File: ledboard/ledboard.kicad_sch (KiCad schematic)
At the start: 45 parts, among them J1 Jack-DC, U1 TPS54332DDA, U2 TPS7A5301BRPSR, U3 TPS2121

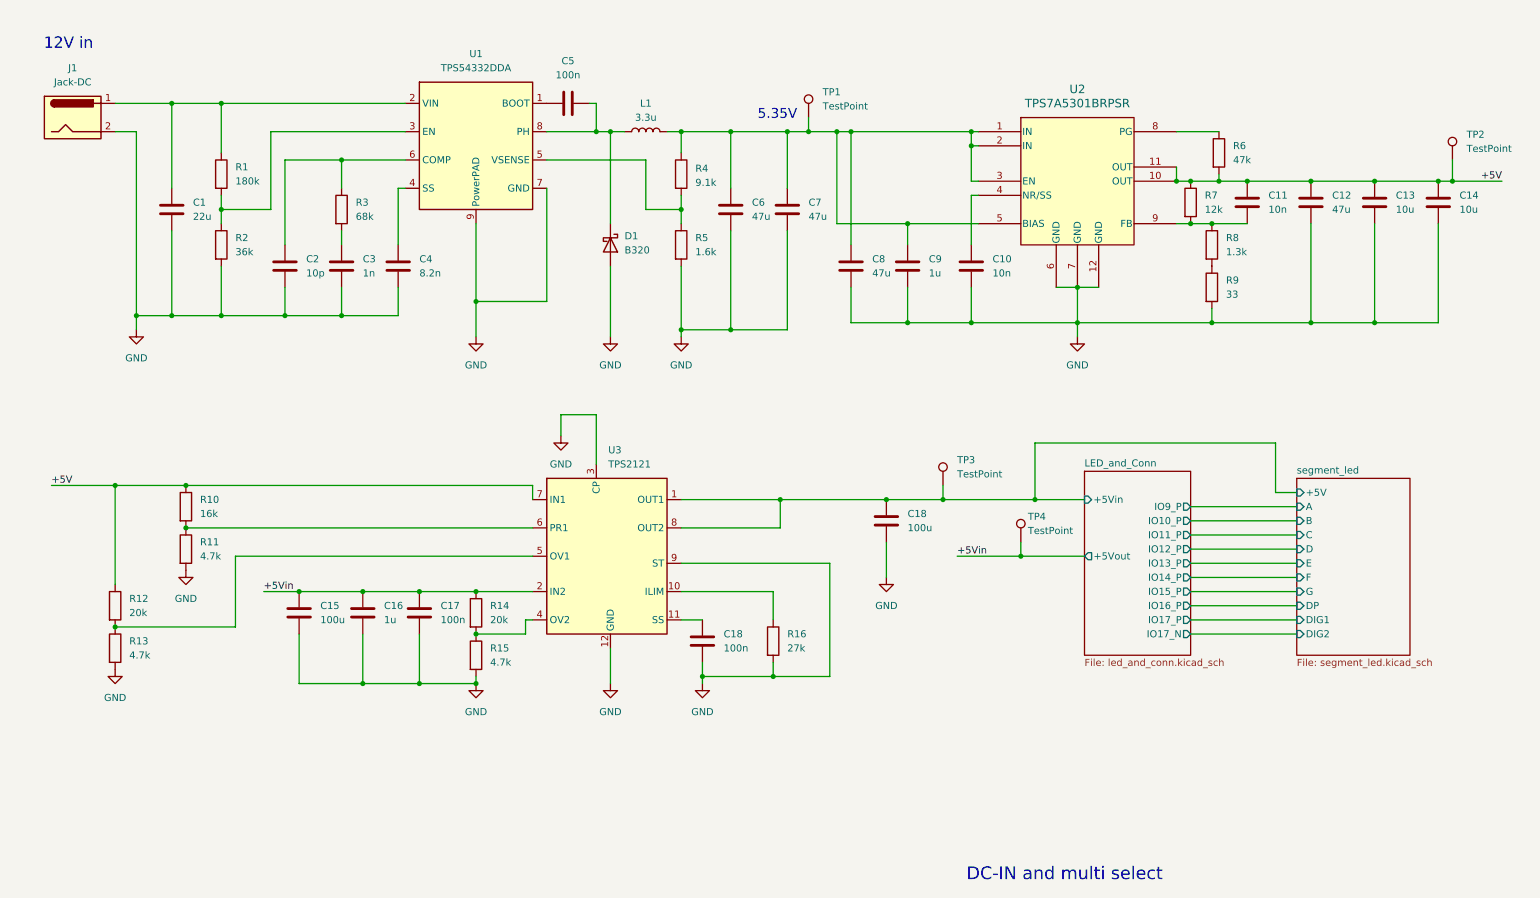
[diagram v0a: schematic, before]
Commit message: 部品が決まったので,コミットします.
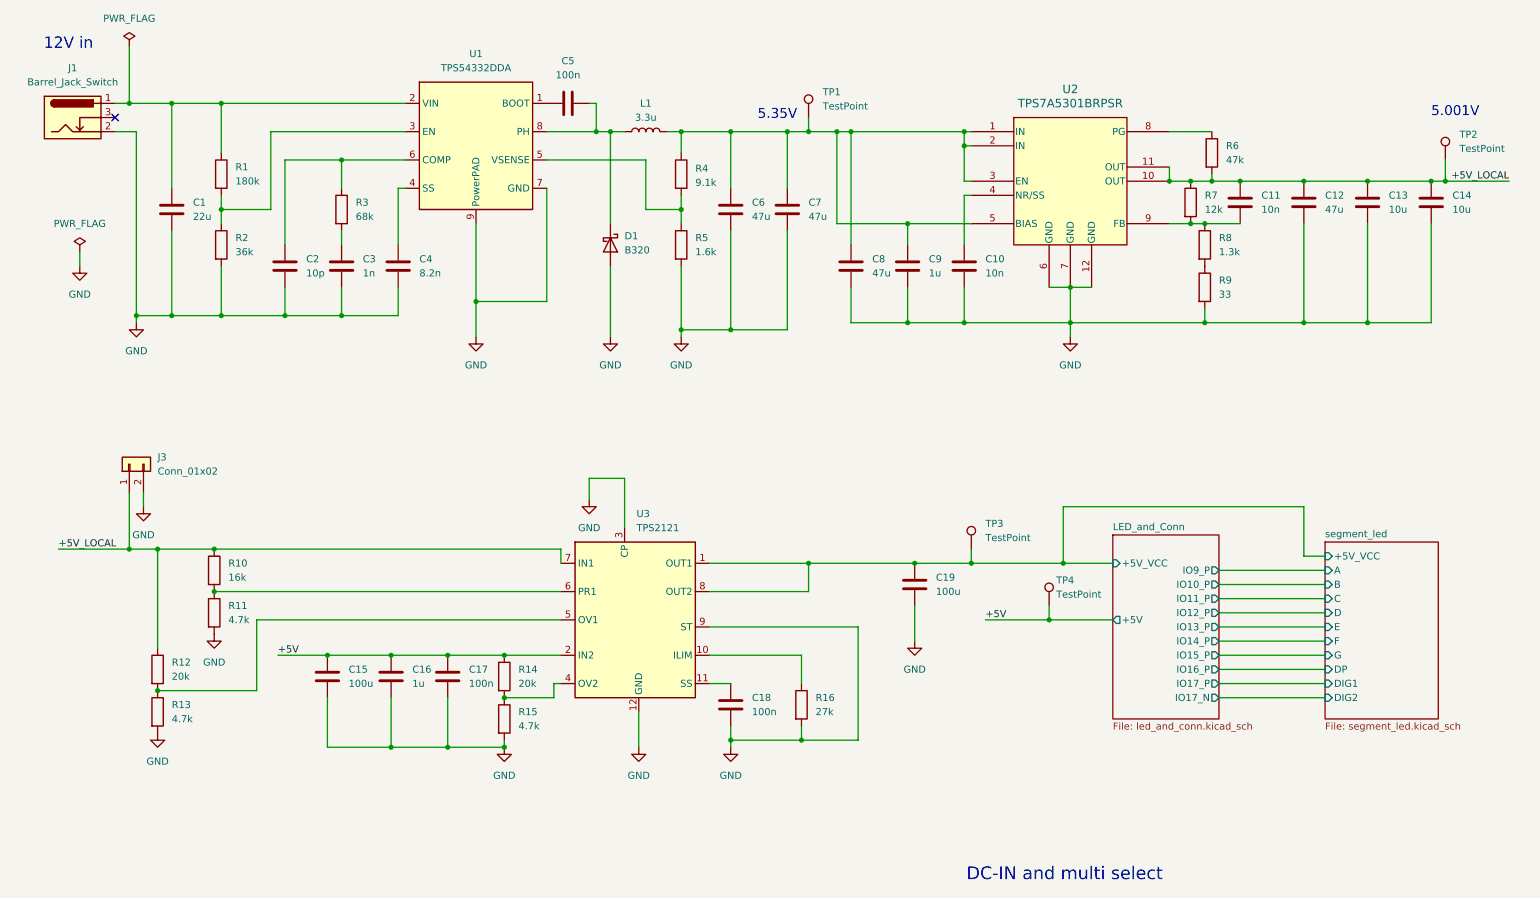
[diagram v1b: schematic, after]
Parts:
- removed J1: Jack-DC, symbol Connector:Jack-DC
- added J1: Barrel_Jack_Switch, MyLib:MPD_EJ503A, symbol Connector:Barrel_Jack_Switch
- added J3: Conn_01x02, Connector_PinHeader_2.54mm:PinHeader_1x02_P2.54mm_Vertical, symbol Connector_Generic:Conn_01x02
- C10: footprint Capacitor_SMD:C_1206_3216Metric -> Capacitor_SMD:C_01005_0402Metric; MPN GRM31CR61C476ME44 -> GRM022R61C103ME01
- C11: footprint (none) -> Capacitor_SMD:C_01005_0402Metric; MPN (none) -> GRM022R61C103ME01; Manufacturer (none) -> Murata
- C12: footprint (none) -> Capacitor_SMD:C_1206_3216Metric; MPN (none) -> GRM31CR61C476ME44; Manufacturer (none) -> Murata
- C13, C14: footprint (none) -> Capacitor_SMD:C_0603_1608Metric; MPN (none) -> GRM188R61C106MA73; Manufacturer (none) -> Murata
- C15: footprint (none) -> Capacitor_SMD:C_1210_3225Metric; MPN (none) -> GRM32ER61A107ME20; Manufacturer (none) -> Murata
- C16: footprint (none) -> Capacitor_SMD:C_0402_1005Metric; MPN (none) -> GRM155C71A105KE11; Manufacturer (none) -> Murata
- C17, C18: footprint (none) -> Capacitor_SMD:C_0201_0603Metric; MPN (none) -> GRM033C81A104ME14; Manufacturer (none) -> Murata
- C19: renamed from C18; footprint (none) -> Capacitor_SMD:C_1210_3225Metric; MPN (none) -> GRM32ER61A107ME20; Manufacturer (none) -> Murata
- C2: MPN GRM1555C2A100JA01 -> GRM0222C1C100JA03
- C3: footprint (none) -> Capacitor_SMD:C_0201_0603Metric; MPN (none) -> GRM033R71C102KA01; Manufacturer (none) -> Murata
- C4: footprint (none) -> Capacitor_SMD:C_0201_0603Metric; MPN (none) -> GRM033B11A822JA01; Manufacturer (none) -> Murata
- C5: footprint (none) -> Capacitor_SMD:C_0201_0603Metric; MPN (none) -> GRM033C81E104ME14; Manufacturer (none) -> Murata
- C9: footprint Capacitor_SMD:C_1206_3216Metric -> Capacitor_SMD:C_0402_1005Metric; MPN GRM31CR61C476ME44 -> GRM155B31C105KA12
- L1: footprint (none) -> MyLib:SPM7054VC-3R3M-D
- R1: MPN (none) -> RC0603FR-07180KL; Manufacturer (none) -> YAGEO
- R10: footprint (none) -> Resistor_SMD:R_0603_1608Metric; MPN (none) -> RC0603FR-0716KL; Manufacturer (none) -> YAGEO
- R11, R13, R15: footprint (none) -> Resistor_SMD:R_0603_1608Metric; MPN (none) -> RC0603FR-074K7L; Manufacturer (none) -> YAGEO
- R12, R14: footprint (none) -> Resistor_SMD:R_0603_1608Metric; MPN (none) -> RC0603FR-0720KL; Manufacturer (none) -> YAGEO
- R16: footprint (none) -> Resistor_SMD:R_0603_1608Metric; MPN (none) -> RC0603FR-0727KL; Manufacturer (none) -> YAGEO
- R2: MPN (none) -> RC0603FR-0736KL; Manufacturer (none) -> YAGEO
- R3: footprint (none) -> Resistor_SMD:R_0603_1608Metric; MPN (none) -> RC0603FR-0768KL; Manufacturer (none) -> YAGEO
- R4: footprint (none) -> Resistor_SMD:R_0603_1608Metric; MPN (none) -> RC0603FR-0769K1L; Manufacturer (none) -> YAGEO
- R5: footprint (none) -> Resistor_SMD:R_0603_1608Metric; MPN (none) -> RC0603FR-071K6L; Manufacturer (none) -> YAGEO
- R6: footprint (none) -> Resistor_SMD:R_0603_1608Metric; MPN (none) -> RC0603FR-0747KL; Manufacturer (none) -> YAGEO
- R7: footprint (none) -> Resistor_SMD:R_0603_1608Metric; MPN (none) -> RC0603FR-0712KL; Manufacturer (none) -> YAGEO
- R8: footprint (none) -> Resistor_SMD:R_0603_1608Metric; MPN (none) -> RC0603FR-071K3L; Manufacturer (none) -> YAGEO
- R9: footprint (none) -> Resistor_SMD:R_0603_1608Metric; MPN (none) -> RC0603FR-0733RL; Manufacturer (none) -> YAGEO
- TP1, TP2, TP3, TP4: footprint (none) -> TestPoint:TestPoint_Keystone_5000-5004_Miniature; MPN (none) -> 5002; Manufacturer (none) -> keystone
- U2: MPN (none) -> TPS7A5301BRPSR; Manufacturer (none) -> TI
- U3: MPN TPS2121 -> TPS2121RUXR
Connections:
- net +5Vin is gone; now on net +5V: C15.1, C16.1, C17.1, R14.1, TP4.1, U3.2 (IN2)
- net +5V: no longer C11.1, C12.1, C13.1, C14.1, R10.1, R12.1, R6.2, R7.1, TP2.1, U2.10 (OUT), U2.11 (OUT), U3.7 (IN1)
- net GND: now also J1.2, J3.2 (Pin_2)
- net at C1.1, R1.1, U1.2 (VIN): now also J1.1
- net LED_and_Conn/+5Vin renamed LED_and_Conn/+5V_VCC
- new net +5V_LOCAL: C11.1, C12.1, C13.1, C14.1, J3.1 (Pin_1), R10.1, R12.1, R6.2, R7.1, TP2.1, U2.10 (OUT), U2.11 (OUT), U3.7 (IN1)
- no-connect marks 0 -> 1
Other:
- sheet LED_and_Conn ports: added +5V, +5V_VCC; removed +5Vin, +5Vout
- sheet segment_led ports: added +5V_VCC; removed +5V
- note added: "5.001V"
- moved on the sheet: C10, C11, C12, C13, C14, C15, C16, C17, C18, C19, R10, R11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

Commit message: ERC解消まで.
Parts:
- U3: MPN TPS2121RUXR -> TPS2121
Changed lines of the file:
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@@
 			)
 		)
-		(property "Datasheet" "https://pim.murata.com/asset/pim4/ceramicCapacitorSMD/GRM022R61E103ME01-01A-JP_PDF_CERAMICCAPACITORSMD?lastModifiedDatetime=20250813135319"
+		(property "Datasheet" "~"
 			(at 233.68 52.07 0)
 			(effects
@@
 			)
 		)
-		(property "Datasheet" "https://www.memoryprotectiondevices.com/datasheets/EJ503A/EJ503A-datasheet.pdf"
+		(property "Datasheet" "~"
 			(at 25.4 37.846 0)
 			(effects
@@
 			)
 		)
-		(property "Datasheet" "https://yageogroup.com/content/datasheet/asset/file/PYU-RC_GROUP_51_ROHS_L"
+		(property "Datasheet" "~"
 			(at 39.37 143.51 0)
 			(effects
@@
 			)
 		)
-		(property "Datasheet" "https://pim.murata.com/asset/pim4/ceramicCapacitorSMD/GRM033B11A222JA01-01A-JP_PDF_CERAMICCAPACITORSMD?lastModifiedDatetime=20250813141149"
+		(property "Datasheet" "~"
 			(at 82.55 63.5 0)
 			(effects
@@
 			)
 		)
-		(property "Datasheet" "https://pim.murata.com/asset/pim4/ceramicCapacitorSMD/GRM155B31C105KA12-01A-JP_PDF_CERAMICCAPACITORSMD?lastModifiedDatetime=20250813144309"
+		(property "Datasheet" "~"
 			(at 173.99 63.5 0)
 			(effects
@@
 			)
 		)
-		(property "Datasheet" "https://pim.murata.com/asset/pim4/ceramicCapacitorSMD/GRM033R71C102KA01-01A-JP_PDF_CERAMICCAPACITORSMD?lastModifiedDatetime=20250813141657"
+		(property "Datasheet" "~"
 			(at 72.39 63.5 0)
 			(effects
@@
 			)
 		)
-		(property "Datasheet" "https://www.keyelco.com/userAssets/file/K75p62.pdf"
+		(property "Datasheet" "~"
 			(at 275.59 44.45 0)
 			(effects
@@
 			)
 		)
-		(property "Datasheet" "https://pim.murata.com/asset/pim4/ceramicCapacitorSMD/GRM033C81A104ME14-01A-JP_PDF_CERAMICCAPACITORSMD?lastModifiedDatetime=20250813141354"
+		(property "Datasheet" "~"
 			(at 142.24 142.24 0)
 			(effects
@@
 			)
 		)
-		(property "Datasheet" "https://yageogroup.com/content/datasheet/asset/file/PYU-RC_GROUP_51_ROHS_L"
+		(property "Datasheet" "~"
 			(at 228.6 43.18 0)
 			(effects
@@
 			)
 		)
-		(property "Datasheet" "https://pim.murata.com/asset/pim4/ceramicCapacitorSMD/GRM32ER61A107ME20-01A-JP_PDF_CERAMICCAPACITORSMD?lastModifiedDatetime=20250813153035"
+		(property "Datasheet" "~"
 			(at 69.85 137.16 0)
 			(effects
@@
 			)
 		)
-		(property "Datasheet" "https://pim.murata.com/asset/pim4/ceramicCapacitorSMD/GRM188R61C106MA73-01A-JP_PDF_CERAMICCAPACITORSMD?lastModifiedDatetime=20250813150719"
+		(property "Datasheet" "~"
 			(at 256.54 52.07 0)
 			(effects
@@
 			)
 		)
-		(property "Datasheet" "https://pim.murata.com/asset/pim4/ceramicCapacitorSMD/GRM022R61E103ME01-01A-JP_PDF_CERAMICCAPACITORSMD?lastModifiedDatetime=20250813135319"
+		(property "Datasheet" "~"
 			(at 184.15 63.5 0)
 			(effects
@@
 			)
 		)
-		(property "Datasheet" "https://www.keyelco.com/userAssets/file/K75p62.pdf"
+		(property "Datasheet" "~"
 			(at 204.47 124.46 0)
 			(effects
@@
 			)
 		)
-		(property "Datasheet" "https://pim.murata.com/asset/pim4/ceramicCapacitorSMD/GRM31CC71E226ME15-01A-JP_PDF_CERAMICCAPACITORSMD?lastModifiedDatetime=20250813152619"
+		(property "Datasheet" "~"
 			(at 41.91 53.34 0)
 			(effects
@@
 			)
 		)
-		(property "Datasheet" "https://yageogroup.com/content/datasheet/asset/file/PYU-RC_GROUP_51_ROHS_L"
+		(property "Datasheet" "~"
 			(at 39.37 135.89 0)
 			(effects
@@
 			)
 		)
-		(property "Datasheet" "https://yageogroup.com/content/datasheet/asset/file/PYU-RC_GROUP_51_ROHS_L"
+		(property "Datasheet" "~"
 			(at 227.33 59.69 0)
 			(effects
@@
 			)
 		)
-		(property "Datasheet" "https://www.keyelco.com/userAssets/file/K75p62.pdf"
+		(property "Datasheet" "~"
 			(at 190.5 114.3 0)
 			(effects
@@
 			)
 		)
-		(property "Datasheet" "https://pim.murata.com/asset/pim4/ceramicCapacitorSMD/GRM188R61C106MA73-01A-JP_PDF_CERAMICCAPACITORSMD?lastModifiedDatetime=20250813150719"
+		(property "Datasheet" "~"
 			(at 267.97 52.07 0)
 			(effects
@@
 			)
 		)
-		(property "Datasheet" "https://pim.murata.com/asset/pim4/ceramicCapacitorSMD/GRM32ER61A107ME20-01A-JP_PDF_CERAMICCAPACITORSMD?lastModifiedDatetime=20250813153035"
+		(property "Datasheet" "~"
 			(at 175.26 120.65 0)
 			(effects
@@
 			)
 		)
-		(property "Datasheet" "https://pim.murata.com/asset/pim4/ceramicCapacitorSMD/GRM31CR61C476ME44-01A-JP_PDF_CERAMICCAPACITORSMD?lastModifiedDatetime=20250813152638"
+		(property "Datasheet" "~"
 			(at 142.24 53.34 0)
 			(effects
@@
 			)
 		)
-		(property "Datasheet" "https://pim.murata.com/asset/pim4/ceramicCapacitorSMD/GRM31CR61C476ME44-01A-JP_PDF_CERAMICCAPACITORSMD?lastModifiedDatetime=20250813152638"
+		(property "Datasheet" "~"
 			(at 152.4 53.34 0)
 			(effects
@@
 			)
 		)
-		(property "Datasheet" "https://pim.murata.com/asset/pim4/ceramicCapacitorSMD/GRM31CR61C476ME44-01A-JP_PDF_CERAMICCAPACITORSMD?lastModifiedDatetime=20250813152638"
+		(property "Datasheet" "~"
 			(at 245.11 52.07 0)
 			(effects
@@
 			)
 		)
-		(property "Datasheet" "https://www.keyelco.com/userAssets/file/K75p62.pdf"
+		(property "Datasheet" "~"
 			(at 161.29 36.83 0)
 			(effects
@@
 			)
 		)
-		(property "Datasheet" "https://yageogroup.com/content/datasheet/asset/file/PYU-RC_GROUP_51_ROHS_L"
+		(property "Datasheet" "~"
 			(at 50.8 59.69 0)
 			(effects
@@
 			)
 		)
-		(property "Datasheet" "https://www.ti.com/jp/lit/ds/symlink/tps54332.pdf?ts=1774599358950&ref_url=https%253A%252F%252Fwww.ti.com%252Fproduct%252Fja-jp%252FTPS54332%253Futm_source%253Dgoogle%2526utm_medium%253Dcpc%2526utm_campaign%253Dapp-null-null-gpn_jp-cpc-pf-google-jp_jp_cons%2526utm_content%253DTPS54332%2526ds_k%253DTPS54332%2526DCM%253Dyes%2526gclsrc%253Daw.ds%2526gad_source%253D1%2526gad_campaignid%253D20279248515%2526gclid%253DCj0KCQjw1ZjOBhCmARIsADDuFTBmD5gUQSDSVcVDqtlcqWftM3LiZUXBOSejrsmSzrKRocTvUMsoHYIaAuFjEALw_wcB"
+		(property "Datasheet" "https://www.ti.com/product/ja-jp/TPS54332#cad-cae-symbols"
 			(at 96.52 41.91 0)
 			(effects
@@
 			)
 		)
-		(property "Description" ""
+		(property "Description" "DC-DC Converter"
 			(at 96.52 41.91 0)
 			(effects
@@
 			)
 		)
-		(property "Datasheet" "https://pim.murata.com/asset/pim4/ceramicCapacitorSMD/GRM155C71A105KE11-01A-JP_PDF_CERAMICCAPACITORSMD?lastModifiedDatetime=20260115145428"
+		(property "Datasheet" "~"
 			(at 81.28 137.16 0)
 			(effects
@@
 			)
 		)
-		(property "Datasheet" "https://yageogroup.com/content/datasheet/asset/file/PYU-RC_GROUP_51_ROHS_L"
+		(property "Datasheet" "~"
 			(at 154.94 142.24 0)
 			(effects
@@
 			)
 		)
-		(property "Datasheet" "https://pim.murata.com/asset/pim4/ceramicCapacitorSMD/GRM033C81A104ME14-01A-JP_PDF_CERAMICCAPACITORSMD?lastModifiedDatetime=20250813141354"
+		(property "Datasheet" "~"
 			(at 91.44 137.16 0)
 			(effects
@@
 			)
 		)
-		(property "Datasheet" "https://pim.murata.com/asset/pim4/ceramicCapacitorSMD/GRM033C81E104ME14-01A-JP_PDF_CERAMICCAPACITORSMD?lastModifiedDatetime=20250813141359"
+		(property "Datasheet" "~"
 			(at 113.03 34.29 0)
 			(effects
@@
 			)
 		)
-		(property "Datasheet" "https://yageogroup.com/content/datasheet/asset/file/PYU-RC_GROUP_51_ROHS_L"
+		(property "Datasheet" "~"
 			(at 101.6 137.16 0)
 			(effects
@@
 			)
 		)
-		(property "Datasheet" "https://yageogroup.com/content/datasheet/asset/file/PYU-RC_GROUP_51_ROHS_L"
+		(property "Datasheet" "~"
 			(at 50.8 46.99 0)
 			(effects
@@
 			)
 		)
-		(property "Datasheet" "https://yageogroup.com/content/datasheet/asset/file/PYU-RC_GROUP_51_ROHS_L"
+		(property "Datasheet" "~"
 			(at 227.33 67.31 0)
 			(effects
@@
 			)
 		)
-		(property "Datasheet" "https://yageogroup.com/content/datasheet/asset/file/PYU-RC_GROUP_51_ROHS_L"
+		(property "Datasheet" "~"
 			(at 224.79 52.07 0)
 			(effects
@@
 			)
 		)
-		(property "Datasheet" "https://yageogroup.com/content/datasheet/asset/file/PYU-RC_GROUP_51_ROHS_L"
+		(property "Datasheet" "~"
 			(at 101.6 144.78 0)
 			(effects
@@
 			)
 		)
-		(property "Datasheet" "https://yageogroup.com/content/datasheet/asset/file/PYU-RC_GROUP_51_ROHS_L"
+		(property "Datasheet" "~"
 			(at 133.35 59.69 0)
 			(effects
@@
 			)
 		)
-		(property "Datasheet" "https://pim.murata.com/asset/pim4/ceramicCapacitorSMD/GRM0222C1C100JA03-01A-JP_PDF_CERAMICCAPACITORSMD?lastModifiedDatetime=20250813133405"
+		(property "Datasheet" "~"
 			(at 62.23 63.5 0)
 			(effects
@@
 			)
 		)
-		(property "Datasheet" "https://yageogroup.com/content/datasheet/asset/file/PYU-RC_GROUP_51_ROHS_L"
+		(property "Datasheet" "~"
 			(at 49.53 118.11 0)
 			(effects
@@
 			)
 		)
-		(property "MPN" "TPS2121RUXR"
+		(property "MPN" "TPS2121"
 			(at 124.46 123.19 0)
 			(effects
@@
 			)
 		)
-		(property "Datasheet" "https://yageogroup.com/content/datasheet/asset/file/PYU-RC_GROUP_51_ROHS_L"
+		(property "Datasheet" "~"
 			(at 133.35 46.99 0)
 			(effects
@@
 			)
 		)
-		(property "Datasheet" "https://product.tdk.com/system/files/dam/doc/product/inductor/inductor/smd/catalog/inductor_automotive_power_spm7054vc-d_en.pdf"
+		(property "Datasheet" "~"
 			(at 127 39.37 0)
 			(effects
@@
 			)
 		)
-		(property "Datasheet" "https://pim.murata.com/asset/pim4/ceramicCapacitorSMD/GRM31CR61C476ME44-01A-JP_PDF_CERAMICCAPACITORSMD?lastModifiedDatetime=20250813152638"
+		(property "Datasheet" "~"
 			(at 163.83 63.5 0)
 			(effects
@@
 			)
 		)
-		(property "Datasheet" "https://www.diodes.com/datasheet/download/B320.pdf"
+		(property "Datasheet" "http://www.jameco.com/Jameco/Products/ProdDS/1538777.pdf"
 			(at 120.65 59.69 0)
 			(effects
@@
 			)
 		)
-		(property "Datasheet" "https://yageogroup.com/content/datasheet/asset/file/PYU-RC_GROUP_51_ROHS_L"
+		(property "Datasheet" "~"
 			(at 72.39 53.34 0)
 			(effects
@@
 			)
 		)
-		(property "Datasheet" "https://yageogroup.com/content/datasheet/asset/file/PYU-RC_GROUP_51_ROHS_L"
+		(property "Datasheet" "~"
 			(at 49.53 125.73 0)
 			(effects

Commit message: 部品変更とアートワークの修正.
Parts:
- C10: footprint Capacitor_SMD:C_01005_0402Metric -> Capacitor_SMD:C_0402_1005Metric; MPN GRM022R61C103ME01 -> GRM155R71C103KA01D
- C2: footprint Capacitor_SMD:C_01005_0402Metric -> Capacitor_SMD:C_0402_1005Metric; MPN GRM0222C1C100JA03 -> GRM1555C1E100JA01D
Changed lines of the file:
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@@
 			)
 		)
-		(property "Footprint" "Capacitor_SMD:C_01005_0402Metric"
+		(property "Footprint" "Capacitor_SMD:C_0402_1005Metric"
 			(at 185.1152 67.31 0)
 			(effects
@@
 			)
 		)
-		(property "MPN" "GRM022R61C103ME01"
+		(property "MPN" "GRM155R71C103KA01D"
 			(at 184.15 63.5 0)
 			(effects
@@
 			)
 		)
-		(property "Footprint" "Capacitor_SMD:C_01005_0402Metric"
+		(property "Footprint" "Capacitor_SMD:C_0402_1005Metric"
 			(at 63.1952 67.31 0)
 			(effects
@@
 			)
 		)
-		(property "MPN" "GRM0222C1C100JA03"
+		(property "MPN" "GRM1555C1E100JA01D"
 			(at 62.23 63.5 0)
 			(effects
